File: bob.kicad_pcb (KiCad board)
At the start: 2 copper layers, 58.4 x 25.4 mm, 52 parts, among them J1 Mini USB Female, J2 GPIO (Optional), J3 GPIO (Optional), J4 Screw Terminal, 2.54mm, J5 Conn_01x04_Male, J6 Conn_01x03_Male, Q1 IRFML8244TRPBF, Q2 IRFML8244TRPBF, U1 W25Q64JVSS, U2 AMS1117-3.3, U3 RP2040, U4 QMI8658C, U5 HP203B, U6 QMC5883L, Y1 12MHz

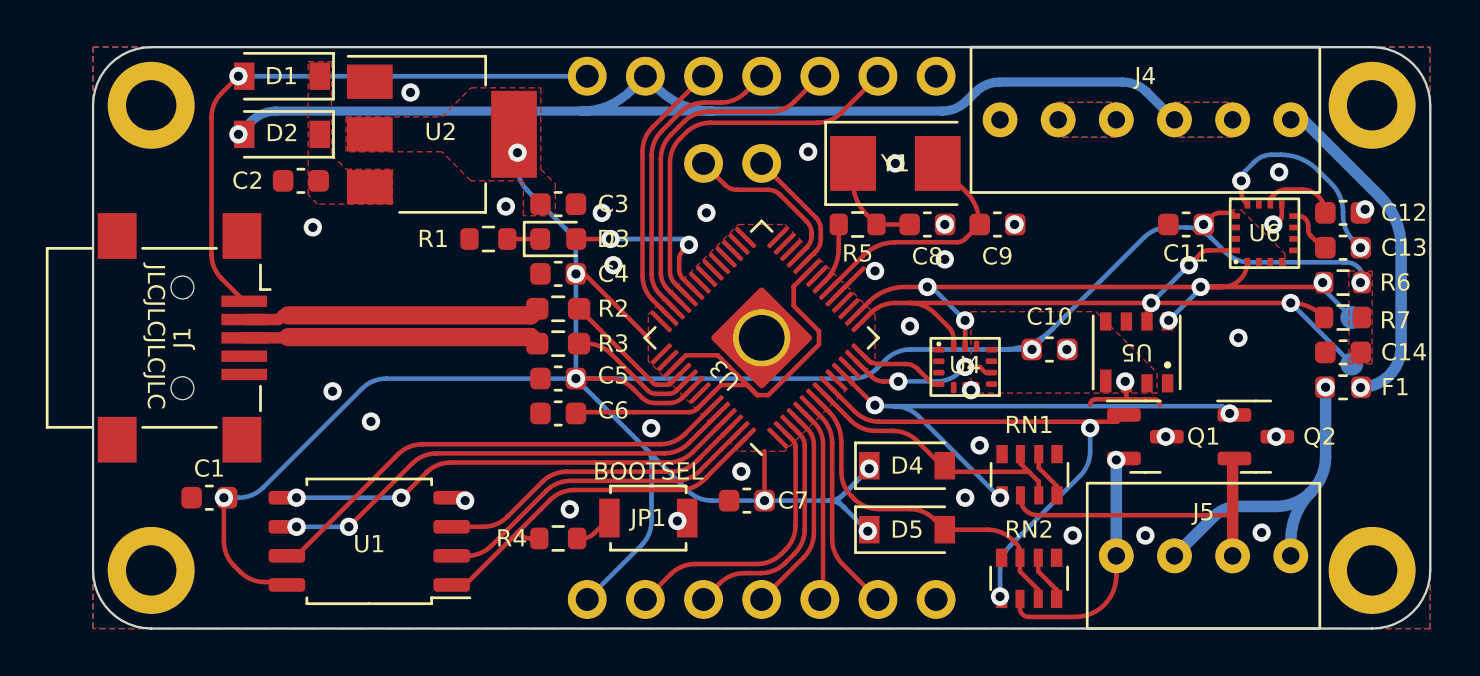
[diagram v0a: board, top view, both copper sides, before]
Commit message: Rev 4 issued for production
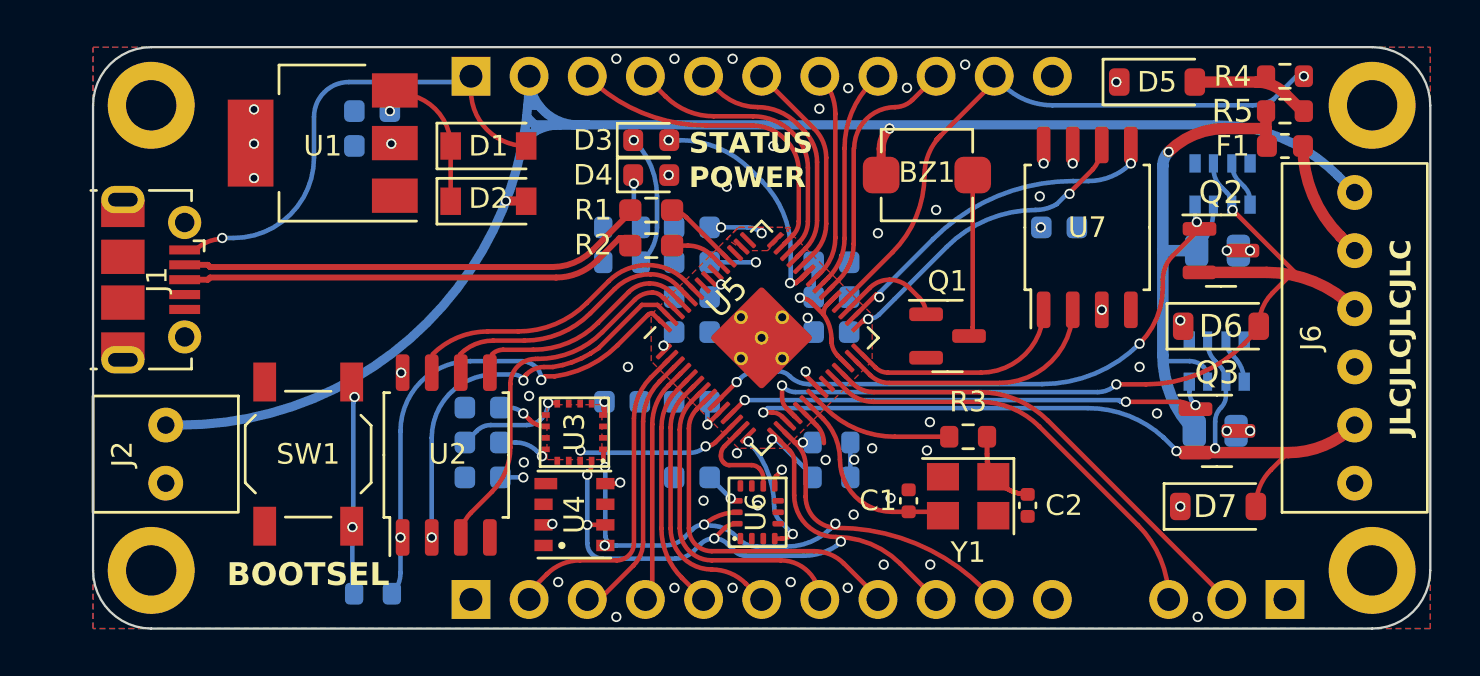
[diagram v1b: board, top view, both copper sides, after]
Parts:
- removed JP1: BOOTSEL, Button_Switch_SMD:SW_SPST_B3U-1000P
- removed TP1, TP2: TestPoint, TestPoint:TestPoint_Pad_D1.0mm
- removed the YAR at (23.4, 30.5)
- added BZ1: Buzzer, YAR_other:Cy-SMD-4020-3040, F.Cu at (50.4, 23.4)
- added C15: 220n, Capacitor_SMD:C_0603_1608Metric, B.Cu at (31.0, 35.1)
- added C16: 100n, Capacitor_SMD:C_0603_1608Metric, B.Cu at (31.0, 36.6)
- added C17: 10u, Capacitor_SMD:C_0603_1608Metric, B.Cu at (26.2, 20.6)
- added C18: 10u, Capacitor_SMD:C_0603_1608Metric, B.Cu at (26.2, 22.1)
- added D6: B5819W SL, Diode_SMD:D_SOD-123, F.Cu at (63.2, 30.0)
- added D7: B5819W SL, Diode_SMD:D_SOD-123, F.Cu at (63.1, 37.8)
- added Q3: AO3400A, Package_TO_SOT_SMD:SOT-23, F.Cu at (63.1, 34.5)
- added R10: 220, Resistor_SMD:R_0603_1608Metric, B.Cu at (37.1, 25.7)
- added R11: 220, Resistor_SMD:R_0603_1608Metric, B.Cu at (37.1, 27.2)
- added R12: 1k, Resistor_SMD:R_0603_1608Metric, B.Cu at (26.2, 41.7)
- added R8: 3k6, Resistor_SMD:R_0603_1608Metric, B.Cu at (46.2, 35.1)
- added R9: 3k6, Resistor_SMD:R_0603_1608Metric, B.Cu at (46.2, 36.6)
- added SW1: Bootsel, Button_Switch_SMD:SW_SPST_TL3342, F.Cu at (23.4, 35.6)
- added U7: W25Q128JVSS, Package_SO:SOIC-8_5.23x5.23mm_P1.27mm, F.Cu at (57.4, 25.7)
- added YAR: LOGO, YAR_Logos:yar_new, B.Cu at (24.1, 27.9)
- C1: value 100n -> 7p; footprint Capacitor_SMD:C_0603_1608Metric -> Capacitor_SMD:C_0402_1005Metric
- C10, C11, C5: moved to B.Cu
- C12: value 4.7u -> 100n; moved to B.Cu
- C13: value 220n -> 100n; moved to B.Cu
- C14: value 100n -> 4.7u; moved to B.Cu
- C2: value 10u -> 7p; footprint Capacitor_SMD:C_0603_1608Metric -> Capacitor_SMD:C_0402_1005Metric
- C3: value 10u -> 100n; moved to B.Cu
- C4, C6: value 1u -> 100n; moved to B.Cu
- C7: value 100n -> 1u; moved to B.Cu
- C8: value 4p -> 1u; moved to B.Cu
- C9: value 4p -> 100n; moved to B.Cu
- D1, D2, D5: value 1N4007 -> B5819W SL
- D3: value RED -> GREEN
- D4: value 1N4007 -> RED; footprint Diode_SMD:D_SOD-123 -> LED_SMD:LED_0603_1608Metric
- J1: value Mini USB Female -> Micro USB Female; footprint Connector_USB:USB_Mini-B_Lumberg_2486_01_Horizontal -> Connector_USB:USB_Micro-B_Molex-105017-0001
- J2: value GPIO (Optional) -> Screw Terminal, 2.54mm; footprint Connector_PinHeader_2.54mm:PinHeader_1x07_P2.54mm_Vertical_NoSilk -> YAR_Connectors:ScrewTerm_2.54x02
- J3: footprint Connector_PinHeader_2.54mm:PinHeader_1x07_P2.54mm_Vertical_NoSilk -> Connector_PinHeader_2.54mm:PinHeader_1x11_P2.54mm_Vertical
- J4: value Screw Terminal, 2.54mm -> GPIO (Optional); footprint YAR_Connectors:ScrewTerm_2.54x06 -> Connector_PinHeader_2.54mm:PinHeader_1x11_P2.54mm_Vertical
- J5: value Conn_01x04_Male -> Conn_01x03_Male; footprint YAR_Connectors:ScrewTerm_2.54x04 -> Connector_PinHeader_2.54mm:PinHeader_1x03_P2.54mm_Vertical
- J6: value Conn_01x03_Male -> Conn_01x06_Pin; footprint Connector_PinHeader_2.54mm:PinHeader_1x02_P2.54mm_Vertical -> YAR_Connectors:ScrewTerm_2.54x06; moved to F.Cu
- Q1, Q2: value IRFML8244TRPBF -> AO3400A
- R1: value 220 -> 27; footprint Resistor_SMD:R_0603_1608Metric -> Resistor_SMD:R_0603_1608Metric_Pad0.98x0.95mm_HandSolder
- R3: value 27 -> 1k; footprint Resistor_SMD:R_0603_1608Metric_Pad0.98x0.95mm_HandSolder -> Resistor_SMD:R_0603_1608Metric
- R4, R5: value 1k -> 3k6
- R6, R7: value 10k -> 4; footprint Resistor_SMD:R_0603_1608Metric -> Resistor_SMD:R_0805_2012Metric; moved to B.Cu
- RN1, RN2: value 22k -> 10k; moved to B.Cu
- U1: value W25Q64JVSS -> AMS1117-3.3; footprint Package_SO:SOIC-8_5.23x5.23mm_P1.27mm -> Package_TO_SOT_SMD:SOT-223-3_TabPin2
- U2: value AMS1117-3.3 -> W25Q128JVSS; footprint Package_TO_SOT_SMD:SOT-223-3_TabPin2 -> Package_SO:SOIC-8_5.23x5.23mm_P1.27mm
- U3: value RP2040 -> QMC5883L; footprint YAR_MCU:RP2040-QFN-56_HS -> YAR_Sensors:QMC5883L-LGA16
- U4: value QMI8658C -> HP203B; footprint YAR_Sensors:QMI8658C-LGA14 -> YAR_Sensors:HP203B-LGA8
- U5: value HP203B -> RP2040; footprint YAR_Sensors:HP203B-LGA8 -> YAR_MCU:RP2040-QFN-56
- U6: value QMC5883L -> QMI8658C; footprint YAR_Sensors:QMC5883L-LGA16 -> YAR_Sensors:QMI8658C-LGA14
- Y1: footprint Crystal:Crystal_SMD_5032-2Pin_5.0x3.2mm -> Crystal:Crystal_SMD_3225-4Pin_3.2x2.5mm
- moved C14 37.7 mm to (31.0, 33.5), turned to 0 degrees
- moved R4 37.6 mm to (66.0, 19.1)
- moved J4 36.2 mm to (30.5, 41.9), turned to 90 degrees
- moved C2 34.8 mm to (54.8, 37.8), turned to 90 degrees
- moved C13 32.2 mm to (37.1, 33.3)
- moved C12 30.7 mm to (40.1, 36.6)
- moved C1 30.6 mm to (49.6, 37.6), turned to -90 degrees
- moved J6 29.5 mm to (69.1, 30.5), turned to 90 degrees
- moved U6 25.3 mm to (43.0, 38.1), turned to -90 degrees
- moved J2 24.7 mm to (17.1, 35.6)
- moved J3 23.4 mm to (30.5, 19.1)
- moved C11 22.9 mm to (40.1, 33.3)
- moved D5 22.4 mm to (60.5, 19.3)
- moved C3 21.9 mm to (56.2, 25.7)
- moved R5 19.3 mm to (66.0, 20.6)
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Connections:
- C1 pad 1: +3V3 -> GND
- C1 pad 2: GND -> Net-(U5-XIN)
- C12 pad 1: GND -> +3V3
- C12 pad 2: Net-(C17-Pad2) -> GND
- C13 pad 1: Net-(C18-Pad1) -> +3V3
- C13 pad 2: Net-(C18-Pad2) -> GND
- C14 pad 1: +3V3 -> GND
- C14 pad 2: GND -> Net-(U3-C1)
- C2 pad 1: Net-(C10-Pad1) -> GND
- C2 pad 2: GND -> Net-(C2-Pad2)
- C8 pad 1: GND -> +1V1
- C8 pad 2: Net-(C13-Pad2) -> GND
- C9 pad 1: GND -> +3V3
- C9 pad 2: XIN -> GND
- D1 pad 1: Net-(C10-Pad1) -> Net-(D1-K)
- D2 pad 1: Net-(C10-Pad1) -> Net-(D1-K)
- D3 pad 1: Net-(D1-Pad1) -> Net-(D3-K)
- D3 pad 2: Net-(D1-Pad2) -> Net-(D3-A)
- D4 pad 1: +3V3 -> Net-(D4-K)
- D4 pad 2: Cont 2 -> +3V3
- D5 pad 2: Cont 1 -> Net-(D5-A)
- F1 pad 1: Net-(F1-Pad1) -> Net-(J6-Pin_5)
- J2 pad 1: VBUS -> GND
- J3 pad 1: +3V3 -> VBUS
- J3 pad 2: GPIO0 -> +BATT
- J3 pad 3: GPIO1 -> GPIO29
- J3 pad 4: GPIO2 -> GPIO28
- J3 pad 5: GPIO3 -> GPIO27
- J3 pad 6: GPIO4 -> GPIO26
- J3 pad 7: GND -> GPIO24
- J4 pad 1: GND -> +3V3
- J4 pad 2: Net-(J2-Pad2) -> GPIO0
- J4 pad 3: Net-(J2-Pad2) -> GPIO1
- J4 pad 4: +BATT -> GPIO2
- J4 pad 5: +BATT -> GPIO3
- J4 pad 6: Net-(F1-Pad1) -> GPIO4
- J5 pad 1: Fire 1 -> GND
- J5 pad 2: ARM -> SWD
- J5 pad 3: Fire 2 -> SWCLK
- J6 pad 1: SWD -> GND
- J6 pad 2: SWCLK -> Cont 2
- Q1 pad 1: Pyro 1 -> BUZZER
- Q1 pad 2: Fire 1 -> GND
- Q1 pad 3: GND -> Net-(BZ1-+)
- Q2 pad 1: Pyro 2 -> Pyro 1
- Q2 pad 2: Fire 2 -> Cont 1
- Q2 pad 3: GND -> Net-(Q2-D)
- R1 pad 1: Net-(D1-Pad1) -> Net-(U5-USB_DM)
- R1 pad 2: GND -> USB_D-
- R2 pad 1: Net-(R2-Pad1) -> Net-(U5-USB_DP)
- R2 pad 2: USB_D- -> USB_D+
- R3 pad 1: Net-(R1-Pad1) -> Net-(C2-Pad2)
- R3 pad 2: USB_D+ -> Net-(U5-XOUT)
- R4 pad 1: Net-(JP1-Pad2) -> ARMED
- R4 pad 2: QSPI_SS -> Net-(D5-A)
- R5 pad 1: Net-(C13-Pad2) -> Net-(D5-A)
- R5 pad 2: XOUT -> ARM
- R6 pad 1: I2C_SCL -> ARM
- R6 pad 2: +3V3 -> Net-(Q2-D)
- R7 pad 1: I2C_SDA -> ARM
- R7 pad 2: +3V3 -> Net-(Q3-D)
- RN1 pad 1: Pyro 2 -> GND
- RN1 pad 2: Fire 2 -> Cont 1
- RN1 pad 3: Cont 2 -> Net-(RN1C-R3.1)
- RN1 pad 4: Net-(RN2-Pad4) -> GND
- RN1 pad 5: GND -> Net-(RN1C-R3.1)
- RN1 pad 6: Net-(RN2-Pad4) -> Cont 1
- RN1 pad 7: Cont 2 -> ARM
- RN1 pad 8: GND -> Pyro 1
- RN2 pad 1: Pyro 1 -> GND
- RN2 pad 2: Fire 1 -> Cont 2
- RN2 pad 3: Cont 1 -> Net-(RN2C-R3.1)
- RN2 pad 4: Net-(RN1-Pad4) -> GND
- RN2 pad 5: GND -> Net-(RN2C-R3.1)
- RN2 pad 6: Net-(RN1-Pad4) -> Cont 2
- RN2 pad 7: Cont 1 -> ARM
- RN2 pad 8: GND -> Pyro 2
- U1 pad 1: QSPI_SS -> GND
- U1 pad 2: QSPI_SD1 -> +3V3
- U1 pad 3: QSPI_SD2 -> Net-(D1-K)
- U2 pad 1: GND -> QSPI_SS
- U2 pad 2: +3V3 -> QSPI_SD1
- U2 pad 3: Net-(C10-Pad1) -> QSPI_SD2
- U3 pad 1: +3V3 -> I2C_SCL
- U3 pad 10: +3V3 -> Net-(U3-C1)
- U3 pad 11: Pyro 2 -> GND
- U3 pad 12: unconnected-(U1-Pad12) -> Net-(U3-SETC)
- U3 pad 13: QMI_INT2 -> +3V3
- U3 pad 14: QMI_INT1 -> (no net)
- U3 pad 15: I2C_SDA -> QMC_DRDY
- U3 pad 16: I2C_SCL -> I2C_SDA
- U3 pad 2: GPIO0 -> +3V3
- U3 pad 3: GPIO1 -> (no net)
- U3 pad 4: GPIO2 -> +3V3
- U3 pad 5: GPIO3 -> (no net)
- U3 pad 6: GPIO4 -> (no net)
- U3 pad 7: Cont 1 -> (no net)
- U3 pad 8: Cont 2 -> Net-(U3-SETP)
- U3 pad 9: Pyro 1 -> GND
- U4 pad 1: GND -> unconnected-(U4-INT1-Pad1)
- U4 pad 3: GND -> +3V3
- U4 pad 4: QMI_INT1 -> (no net)
- U4 pad 5: (no net) -> I2C_SCL
- U4 pad 6: GND -> I2C_SDA
- U4 pad 7: GND -> unconnected-(U4-INT0-Pad7)
- U5 pad 1: unconnected-(U5-Pad1) -> +3V3
- U5 pad 2: GND -> GPIO0
- U5 pad 3: +3V3 -> GPIO1
- U5 pad 4: (no net) -> GPIO2
- U5 pad 5: I2C_SCL -> GPIO3
- U5 pad 6: I2C_SDA -> GPIO4
- U5 pad 7: unconnected-(U5-Pad7) -> GPIO5
- U5 pad 8: +3V3 -> GPIO6
- U6 pad 1: I2C_SCL -> GND
- U6 pad 10: Net-(C17-Pad2) -> (no net)
- U6 pad 11: GND -> (no net)
- U6 pad 12: Net-(C18-Pad2) -> +3V3
- U6 pad 13: +3V3 -> I2C_SCL
- U6 pad 14: (no net) -> I2C_SDA
- U6 pad 2: +3V3 -> GND
- U6 pad 3: (no net) -> GND
- U6 pad 4: +3V3 -> QMI_INT1
- U6 pad 6: (no net) -> GND
- U6 pad 7: (no net) -> GND
- U6 pad 8: Net-(C18-Pad1) -> +3V3
- U6 pad 9: GND -> QMI_INT2
- Y1 pad 1: Net-(C13-Pad2) -> Net-(C2-Pad2)
- Y1 pad 2: XIN -> GND
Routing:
- net +3V3: track 117.1 -> 18.4 mm, vias 10 -> 27
- net ARMED: track 0.00 -> 26.2 mm, vias 0 -> 1
- net Cont 1: track 15.3 -> 39.2 mm, vias 0 -> 3
- net Cont 2: track 12.4 -> 35.9 mm, vias 0 -> 3
- net +BATT: track 48.9 -> 70.9 mm, vias 1 -> 2
- net +1V1: track 20.7 -> 2.02 mm, vias 0 -> 2
- net GPIO6: track 0.00 -> 15.7 mm
- net Net-(F1-Pad1): track 15.0 -> 0.00 mm, vias 1 -> 0
- net SPI_TX: track 0.00 -> 14.5 mm, vias 0 -> 2
- net Fire 2: track 14.1 -> 0.00 mm
- net GPIO5: track 0.00 -> 14.0 mm
- net SPI_SCLK: track 0.00 -> 13.7 mm, vias 0 -> 2
- net SWCLK: track 5.67 -> 19.1 mm
- net SWD: track 7.31 -> 20.6 mm
- net XIN: track 11.6 -> 0.00 mm
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- added copper zone on F.Cu, net +1V1
- added copper zone on In1.Cu, net +3V3
- added copper zone on In2.Cu, net GND
- removed copper zone on F.Cu, net +BATT
- removed copper zone on F.Cu, net Net-(C10-Pad1)
- removed copper zone on B.Cu, net Net-(J2-Pad2)
- removed copper zone on F.Cu, net Net-(J2-Pad2)
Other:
- copper layers 2 -> 4
- board text added: "00"
- board text added: "01"
- board text added: "02"
- board text added: "03"
- board text added: "04"
- board text added: "05"
- board text added: "06"
- board text added: "12V MAX"
- board text added: "22"
- board text added: "23"
- board text added: "24"
- board text added: "3v3"
- board text added: "ARMED"
- board text added: "Bob Rev 4A Claire H 2023"
- board text added: "DRG"
- board text added: "MAIN"
- board text added: "POWER"
- board text added: "STATUS"
- board text added: "VBAT"
- board text added: "VBUS"
- board text removed: "+ -"
- board text removed: "0"
- board text removed: "1"
- board text removed: "2"
- board text removed: "3"
- board text removed: "3V3"
- board text removed: "4"
- board text removed: "BAT"
- board text removed: "BUS"
- board text removed: "Bob Rev 4"
- board text removed: "PYRO 1"
- board text removed: "PYRO 2"
- board text removed: "SWITCH"
- board text removed: "Sensitive Crystal Do not route underneath"
- board text removed: "USB Requires GND underneath"
- board text removed: "X"
- board text removed: "Y"
- board text removed: "Z"
